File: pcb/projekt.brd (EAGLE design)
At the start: 12 parts

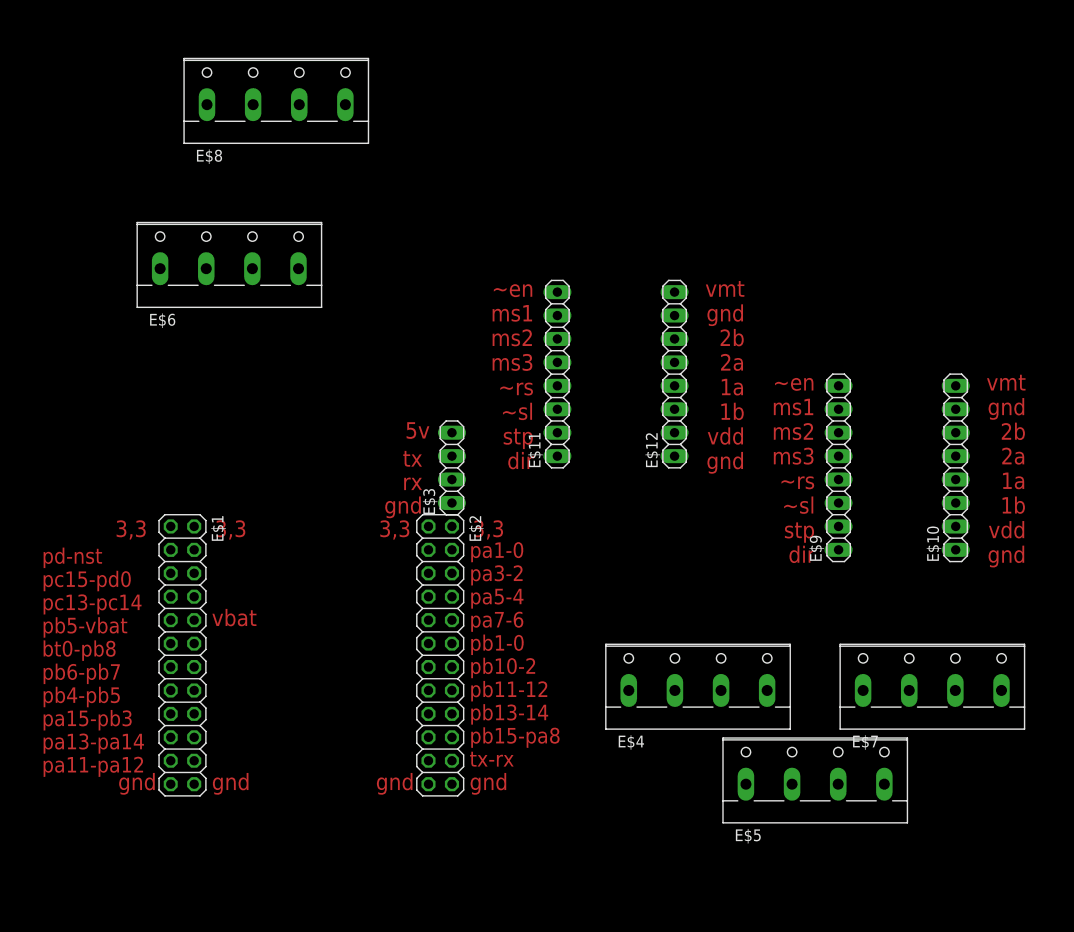
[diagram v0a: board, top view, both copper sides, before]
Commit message: 'pcb_script'
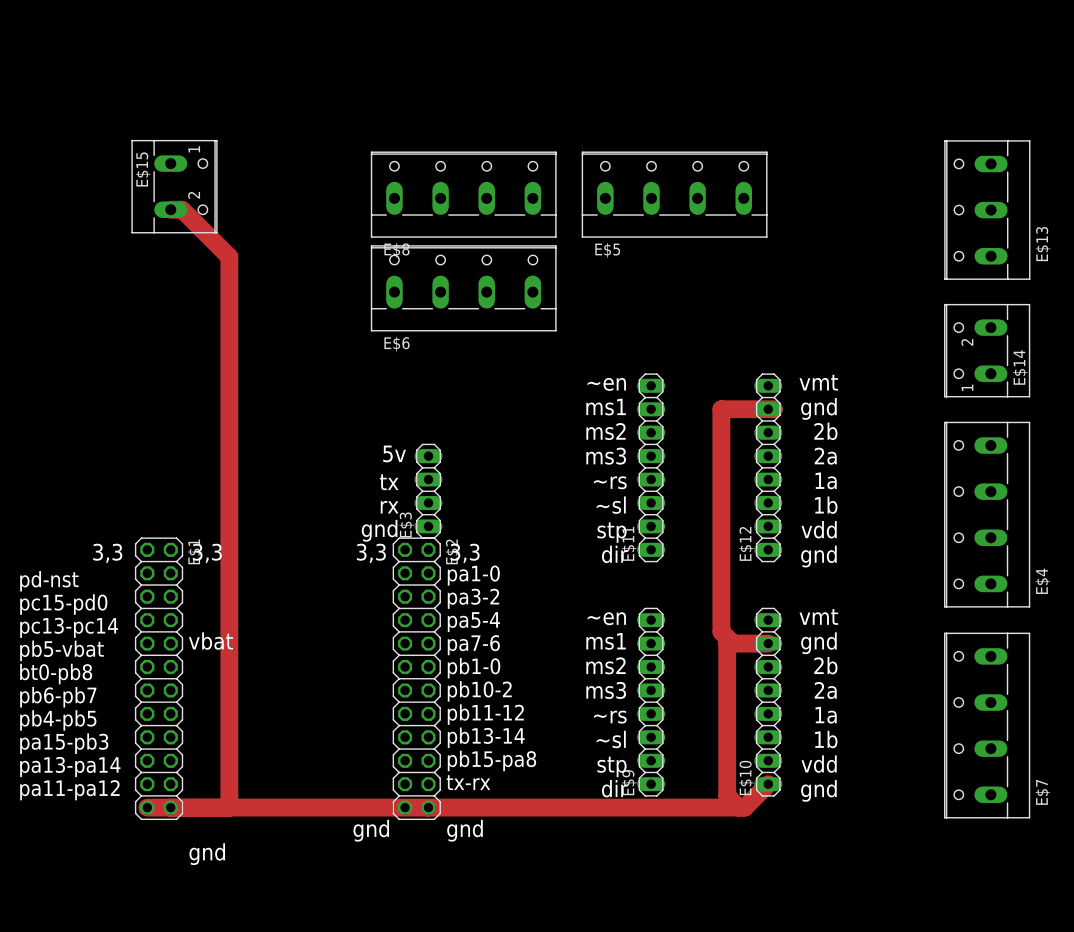
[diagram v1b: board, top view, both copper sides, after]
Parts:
- added E$13: (no value), con-wago-500:W237-103
- added E$14, E$15: (no value), con-wago-500:W237-102
- moved E$5 65.3 mm to (58.4, 68.6)
- moved E$4 35.3 mm to (91.4, 33.0), turned to 90 degrees
- moved E$10 32.5 mm to (68.6, 12.7)
- moved E$9 32.5 mm to (55.9, 12.7)
- moved E$6 25.5 mm to (35.6, 58.4)
- moved E$8 22.7 mm to (35.6, 68.6)
- moved E$11 14.4 mm to (55.9, 38.1)
- moved E$12 14.4 mm to (68.6, 38.1)
- moved E$7 7.18 mm to (91.4, 10.2), turned to 90 degrees
- moved E$2 3.59 mm to (30.5, 15.2)
- moved E$1 3.59 mm to (2.54, 15.2)
- moved E$3 3.59 mm to (31.8, 35.6)
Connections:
- new net S$1: E$1.23, E$1.24, E$15.2, E$2.23, E$2.24
- new net S$2: E$12.1, E$12.7
- new net S$5: E$10.1, E$10.7
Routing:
- net S$1: track 0.00 -> 197.3 mm

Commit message: 'pcb_rotate'
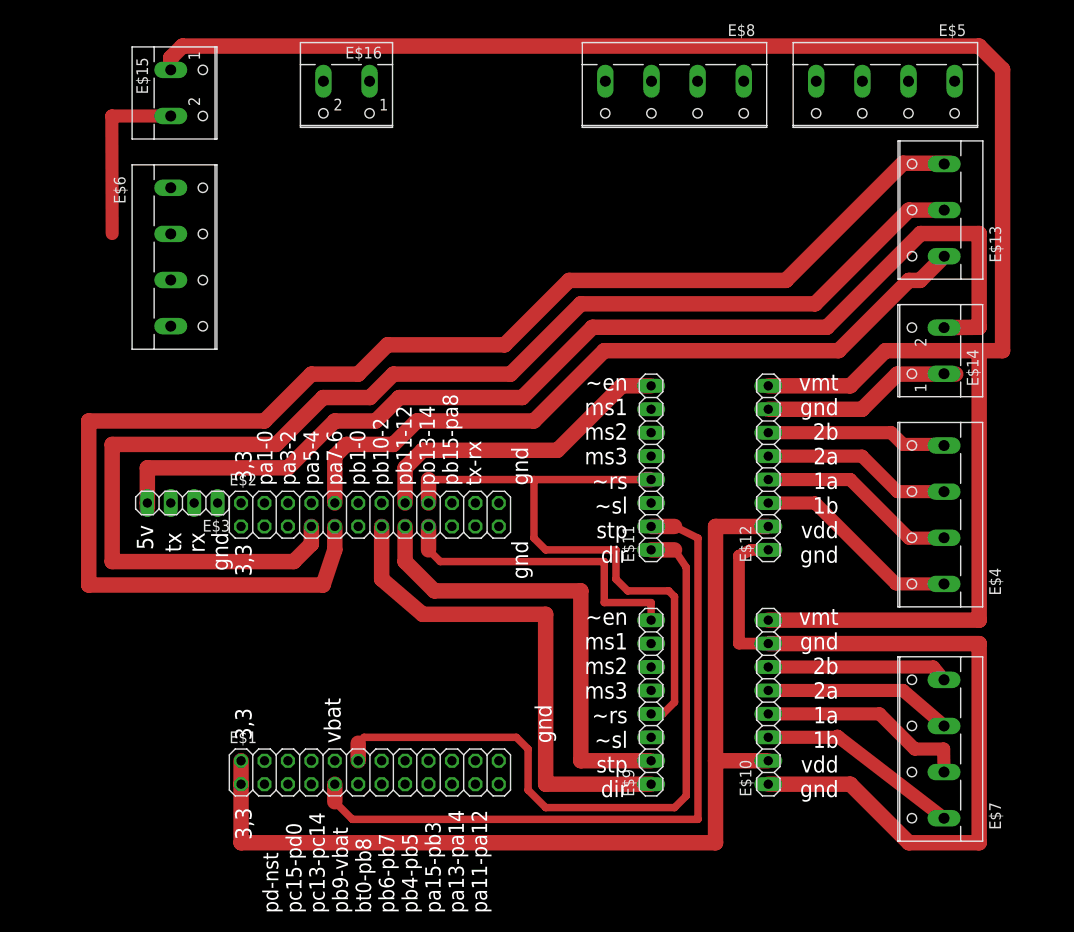
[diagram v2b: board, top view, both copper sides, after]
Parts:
- added E$16: (no value), con-wago-500:W237-102
- moved E$6 30.6 mm to (5.08, 61.0), turned to 270 degrees
- moved E$3 26.7 mm to (5.08, 34.3), turned to 180 degrees
- moved E$1 25.0 mm to (25.4, 5.08), turned to 0 degrees
- moved E$5 25.0 mm to (81.3, 78.7), turned to 180 degrees
- moved E$8 25.0 mm to (58.4, 78.7), turned to 180 degrees
- moved E$2 18.5 mm to (25.4, 33.0), turned to 0 degrees
- moved E$15 10.2 mm to (5.08, 78.7)
- moved E$7 5.68 mm to (86.4, 7.62)
- moved E$13 5.08 mm to (86.4, 66.0)
- moved E$14 5.08 mm to (86.4, 50.8)
- moved E$4 5.08 mm to (86.4, 33.0)
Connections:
- new net S$10: E$1.9, E$11.2
- new net S$11: E$11.8, E$2.16
- new net S$12: E$13.1, E$2.10
- new net S$13: E$13.3, E$2.9
- new net S$14: E$1.10, E$16.2
- new net S$15: E$10.8, E$12.8, E$15.1
- new net S$16: E$1.1, E$1.2, E$10.2, E$12.2
- new net S$17: E$11.4, E$2.18, E$9.4
- new net S$18: E$1.12, E$11.1
- new net S$19: E$13.2, E$2.7
- new net S$20: E$2.13, E$9.1
- new net S$21: E$2.15, E$9.2
- new net S$22: E$2.17, E$9.8
- new net S$23: E$14.2, E$3.4
- new net S$24: E$1.23, E$1.24, E$10.1, E$10.7, E$12.1
- new net S$3: E$10.4, E$7.2
- new net S$4: E$10.5, E$7.3
- new net S$6: E$12.3, E$4.1
- new net S$7: E$12.4, E$4.2
- new net S$8: E$12.5, E$4.3
- new net S$9: E$12.6, E$4.4
- net S$1: now also E$12.7, E$14.1, E$16.1; no longer E$1.23, E$1.24, E$2.23, E$2.24
- net S$2: now also E$10.3, E$7.1; no longer E$12.1, E$12.7
- net S$5: now also E$10.6, E$7.4; no longer E$10.1, E$10.7
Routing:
- net S$15: track 0.00 -> 202.6 mm
- net S$1: track 197.3 -> 41.1 mm
- net S$13: track 0.00 -> 154.7 mm
- net S$19: track 0.00 -> 137.7 mm
- net S$23: track 0.00 -> 119.1 mm
- net S$16: track 0.00 -> 106.0 mm
- net S$24: track 0.00 -> 86.0 mm
- net S$12: track 0.00 -> 80.1 mm
- net S$10: track 0.00 -> 77.9 mm
- net S$18: track 0.00 -> 73.6 mm
- net S$17: track 0.00 -> 67.9 mm
- net S$20: track 0.00 -> 54.7 mm
- net S$21: track 0.00 -> 50.2 mm
- net S$11: track 0.00 -> 34.2 mm
- net S$22: track 0.00 -> 33.5 mm
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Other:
- board text added: "pd-nst pc15-pd0 pc13-pc14 pb9-vbat bt0-pb8 pb6-pb7 pb4-pb5 pa15-pb3 pa13-pa14 pa11-pa12"
- board text removed: "pd-nst pc15-pd0 pc13-pc14 pb5-vbat bt0-pb8 pb6-pb7 pb4-pb5 pa15-pb3 pa13-pa14 pa11-pa12"
